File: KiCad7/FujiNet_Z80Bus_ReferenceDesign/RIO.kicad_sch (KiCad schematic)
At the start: 6 parts

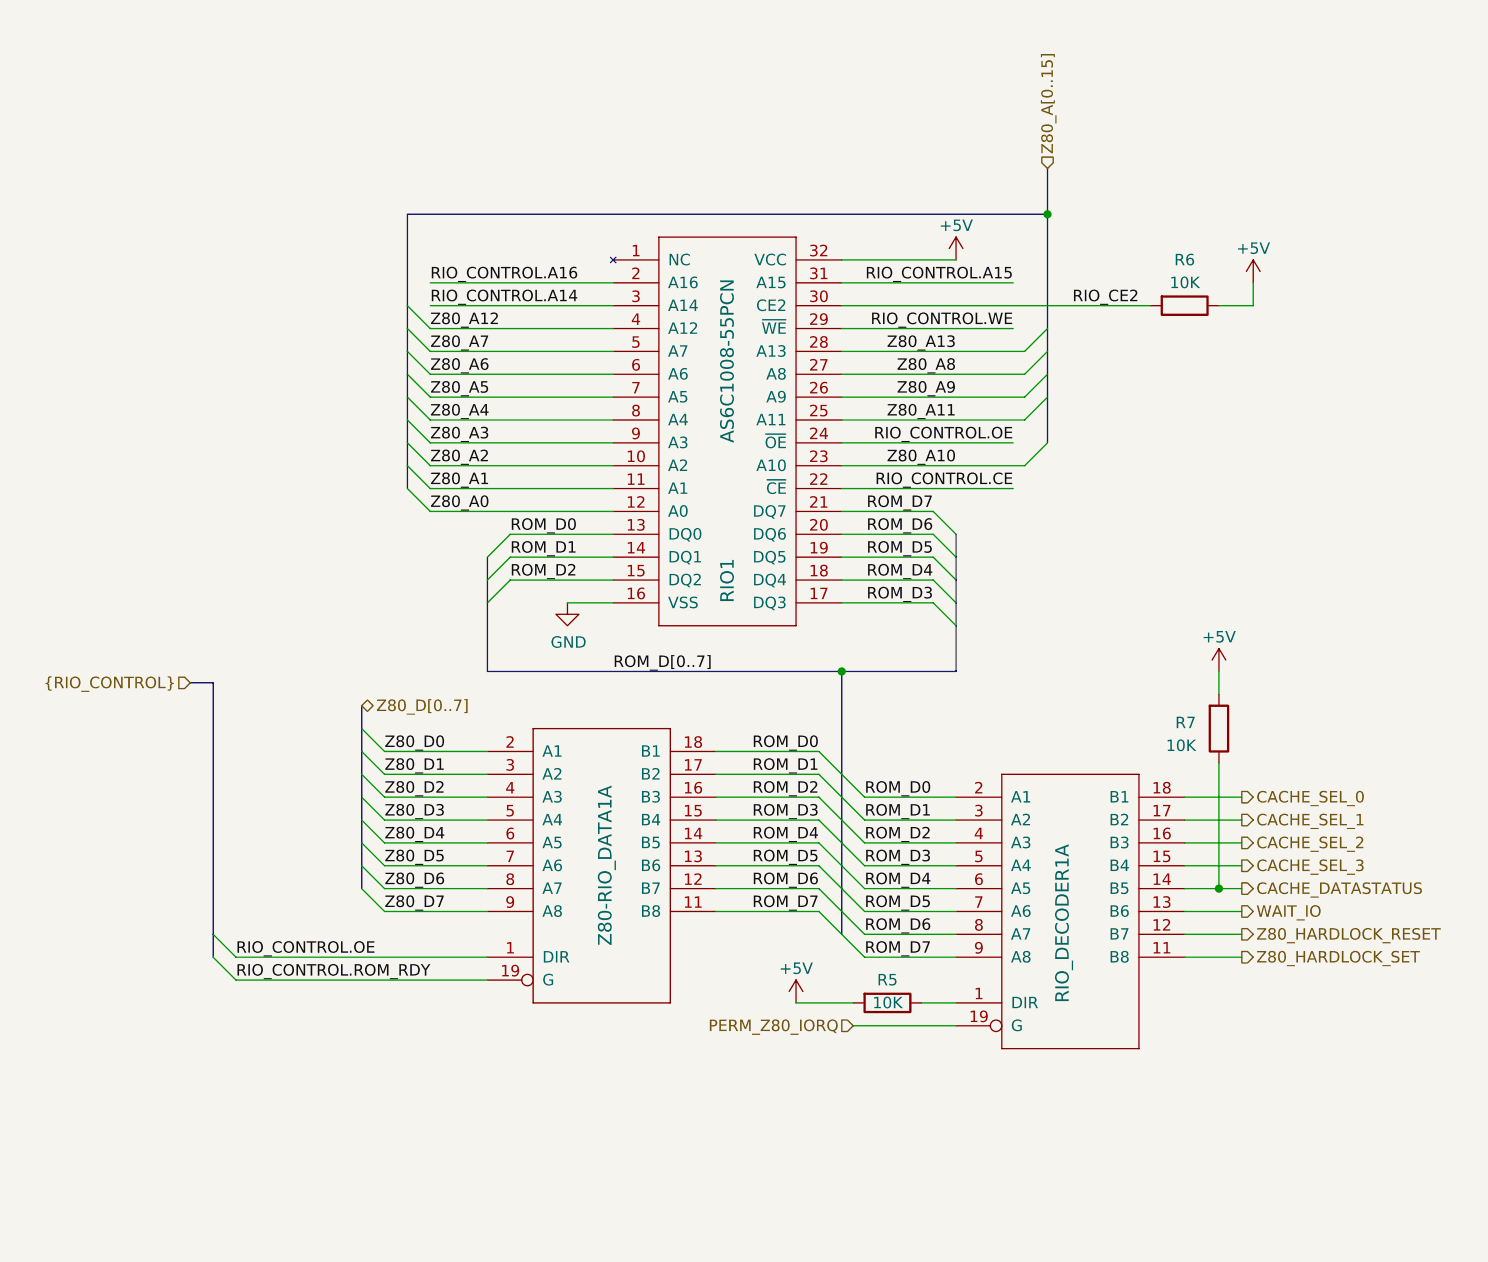
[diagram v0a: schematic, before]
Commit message: KiCad - ALMOST ERROR FREE!!!!
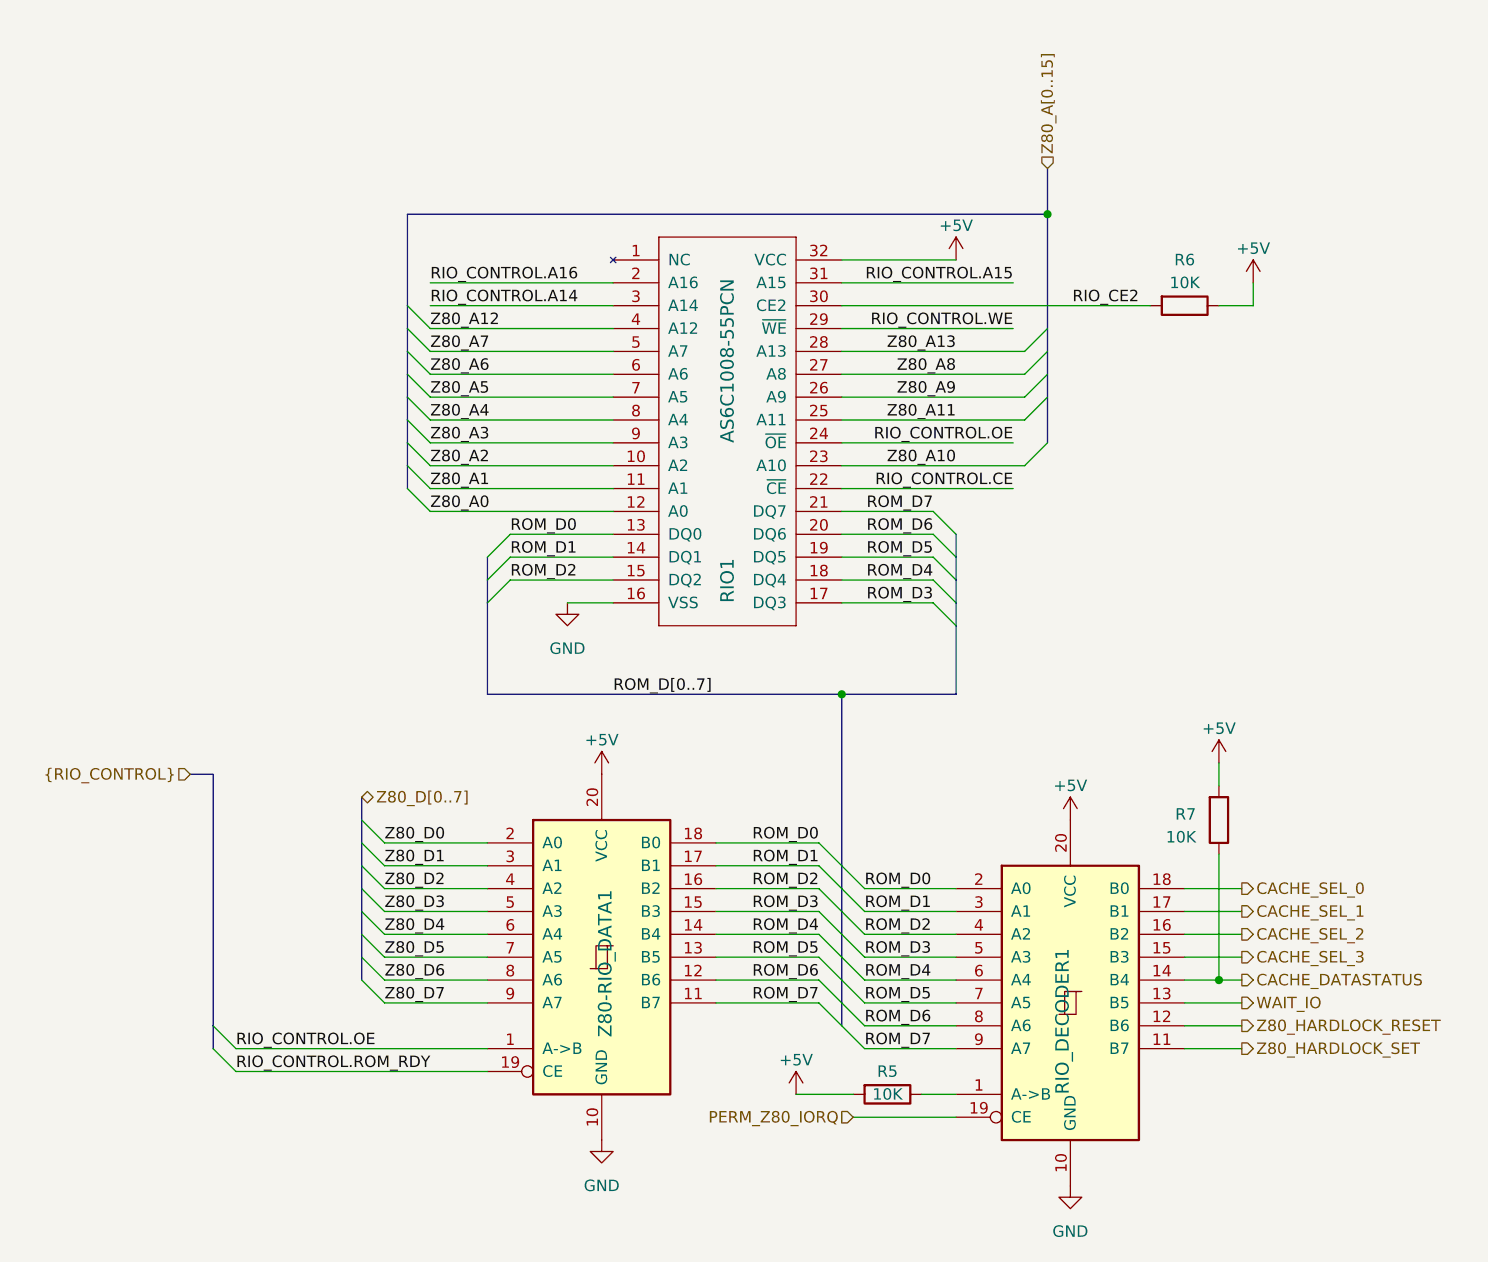
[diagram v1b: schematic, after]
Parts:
- RIO_DECODER1, Z80-RIO_DATA1: symbol FujiNet_Z80Bus_Reference-rescue:74245N-Z80Decoder-eagle-import -> 74xx:74HC245
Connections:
- net +5V: now also RIO_DECODER1.20 (VCC), Z80-RIO_DATA1.20 (VCC)
- net GND: now also RIO_DECODER1.10 (GND), Z80-RIO_DATA1.10 (GND)
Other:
- moved on the sheet: R5, R7
